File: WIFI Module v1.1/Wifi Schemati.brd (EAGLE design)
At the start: 90.1 x 63.4 mm, 26 parts, among them IC1 PIC24FVXXKA302-SP

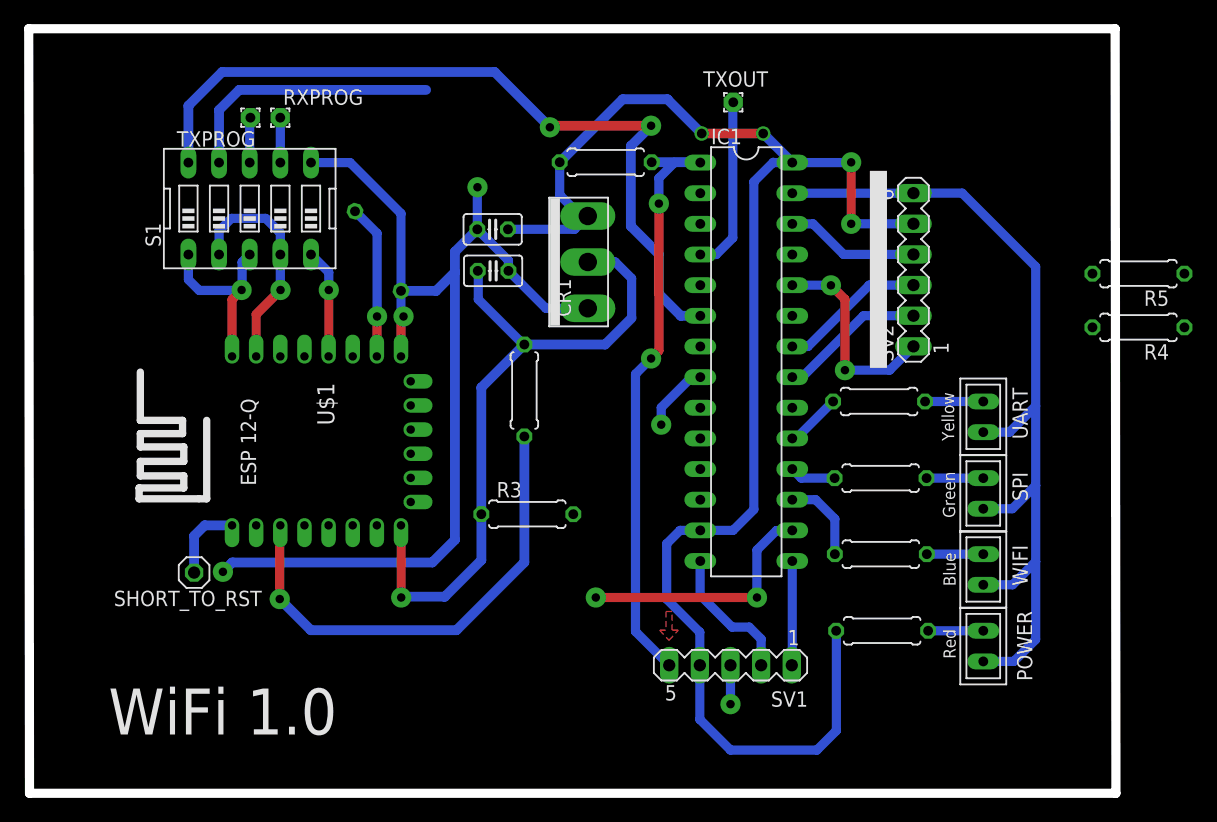
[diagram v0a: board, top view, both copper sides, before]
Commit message: v1.1 PCB Changes
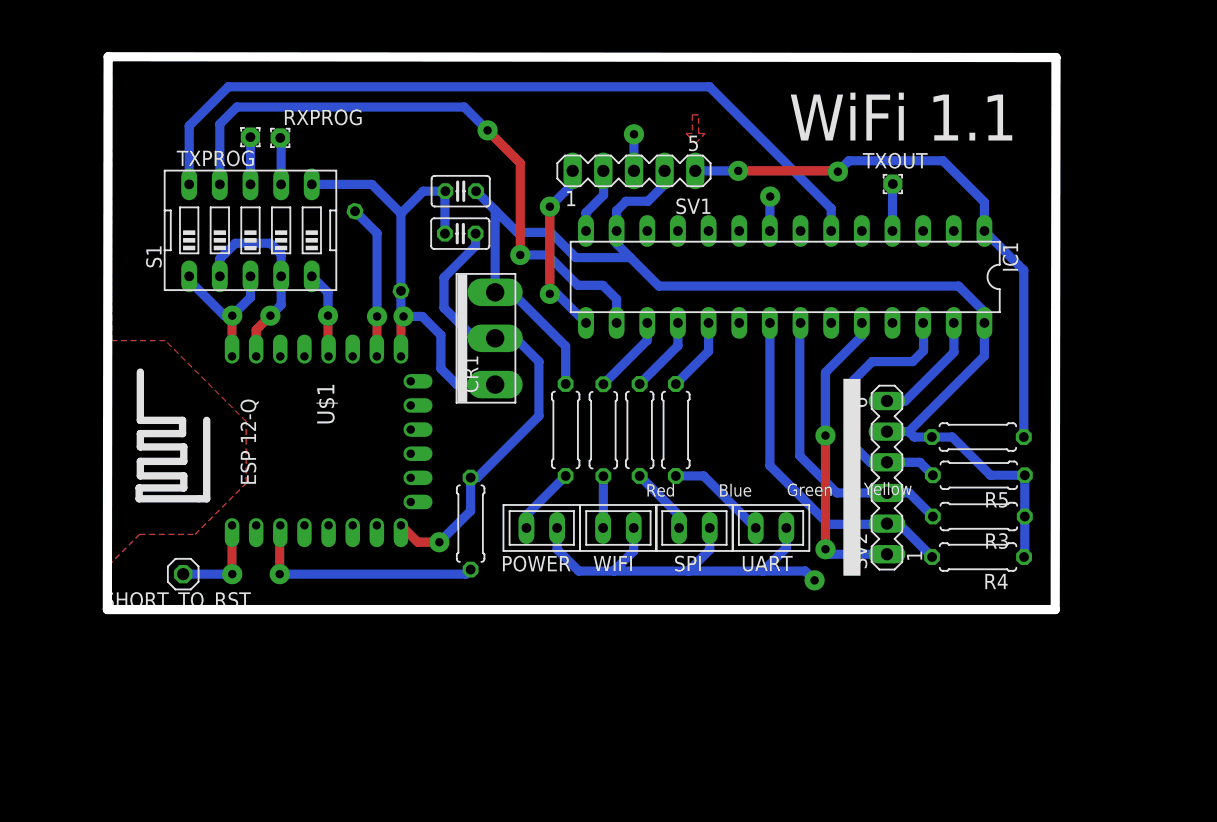
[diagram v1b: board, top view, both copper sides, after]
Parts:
- moved SV1 41.7 mm to (43.7, 15.7), turned to 0 degrees
- moved R1 38.3 mm to (72.2, -6.31)
- moved POWER 37.9 mm to (36.1, -13.9), turned to 0 degrees
- moved R3 37.4 mm to (72.3, -12.9), turned to 180 degrees
- moved RED_POWER 31.1 mm to (38.1, -5.73), turned to 90 degrees
- moved WIFI 30.4 mm to (42.5, -13.9), turned to 0 degrees
- moved BLUE_WIFI 25.2 mm to (41.2, -5.75), turned to 270 degrees
- moved SPI 24.1 mm to (48.8, -13.9), turned to 0 degrees
- moved R4 23.2 mm to (72.3, -16.3)
- moved R5 21.3 mm to (72.3, -9.48)
- moved GREEN_SPI 20.4 mm to (44.2, -5.73), turned to 270 degrees
- moved UART 19.9 mm to (55.1, -13.9), turned to 0 degrees
- moved SV2 17.4 mm to (64.7, -9.68)
- moved YELLOW_UART 17.0 mm to (47.2, -5.73), turned to 270 degrees
- moved TXOUT 14.9 mm to (65.2, 14.7)
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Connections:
- removed net N$12: R4.1, R5.1
- net 3.3V: no longer R3.1
- net VDD: now also R3.1, R4.1, R5.1
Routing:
- net GND: track 172.2 -> 92.6 mm, vias 5 -> 4
- net VDD: track 127.9 -> 106.5 mm, vias 4 -> 0
- net N$6: track 40.2 -> 20.0 mm
- net 3.3V: track 58.4 -> 39.4 mm
- net MOSI: track 12.8 -> 28.5 mm
- net CLK: track 12.2 -> 24.2 mm
- net SS: track 11.1 -> 22.2 mm
- net TXOUT: track 14.5 -> 3.90 mm
- net TXPIC: track 43.1 -> 51.5 mm
- net MISO: track 17.2 -> 25.3 mm
- net PGC: track 8.65 -> 15.0 mm, vias 0 -> 2
- net PGD: track 11.6 -> 5.59 mm
- net MCLR: track 50.4 -> 46.6 mm
- net TX: track 16.0 -> 12.4 mm
- net N$10: track 4.83 -> 8.41 mm
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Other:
- board size 90.1 x 63.4 mm -> 78.6 x 45.8 mm
- board text added: "WiFi 1.1"
- board text removed: "GND"
- board text removed: "WiFi 1.0"
